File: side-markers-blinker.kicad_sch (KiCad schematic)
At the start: 36 parts, among them J1 Conn_01x07_Socket, Q1 BC547, Q2 BC547, Q3 BC547, Q4 BC547, Q5 BC547, Q6 BC547, Q7 IRF4905, Q8 IRF4905

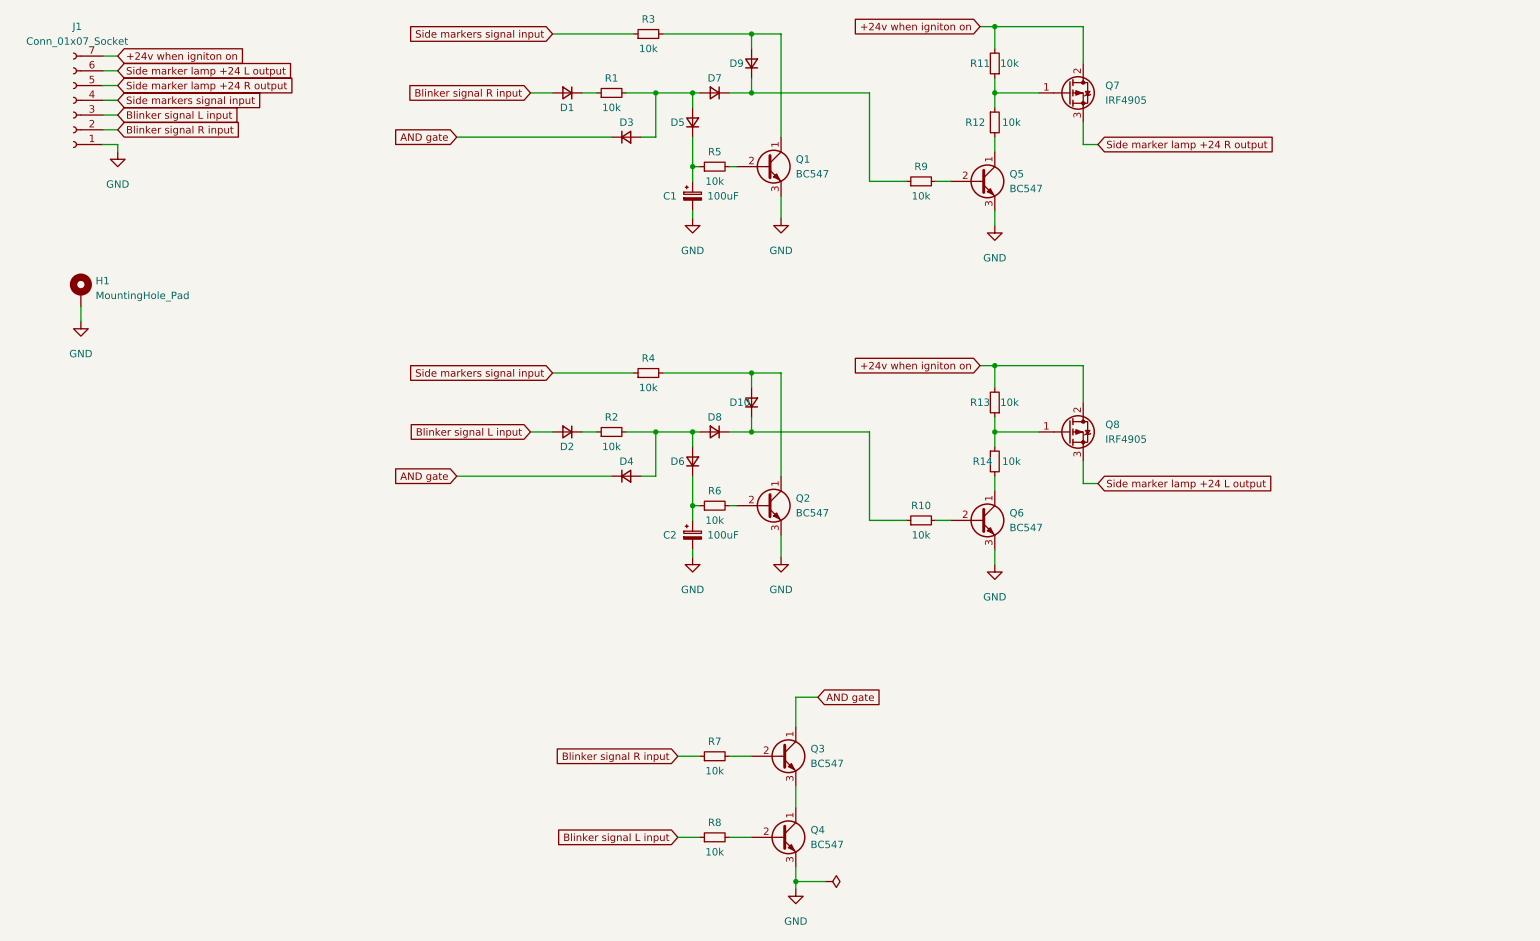
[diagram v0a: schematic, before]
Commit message: Updated schematic.
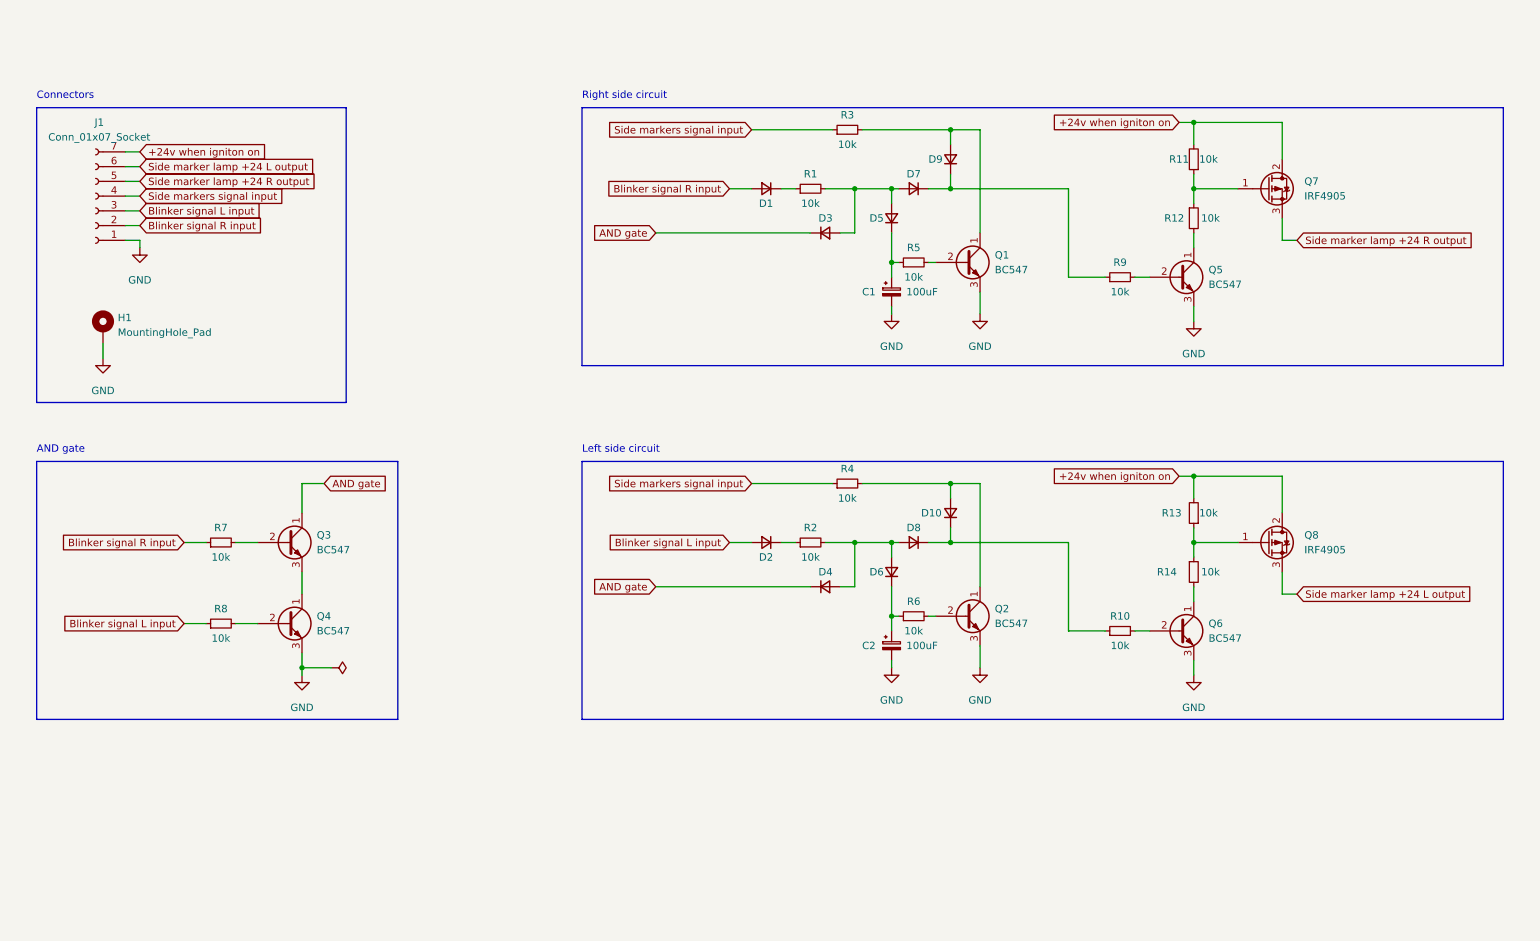
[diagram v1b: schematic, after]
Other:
- note added: "AND gate"
- note added: "Connectors"
- note added: "Left side circuit"
- note added: "Right side circuit"
- moved on the sheet: C1, C2, D1, D10, D2, D3, D4, D5, D6, D7, D8, D9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
